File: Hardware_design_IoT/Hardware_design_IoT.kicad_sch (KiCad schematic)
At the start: 0 parts

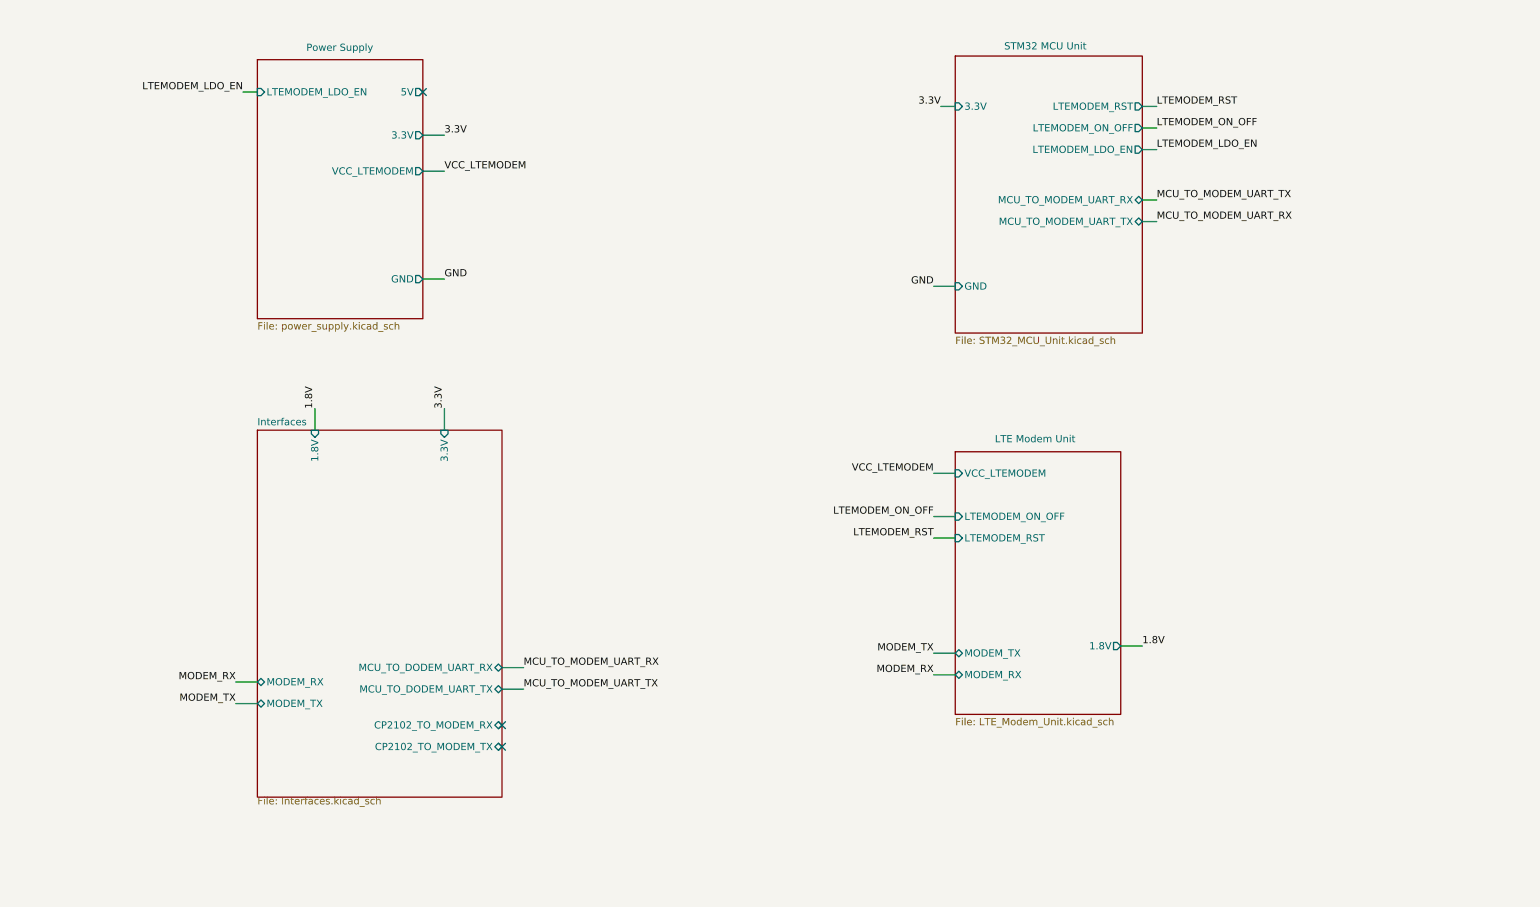
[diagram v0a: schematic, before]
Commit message: Fin du projet
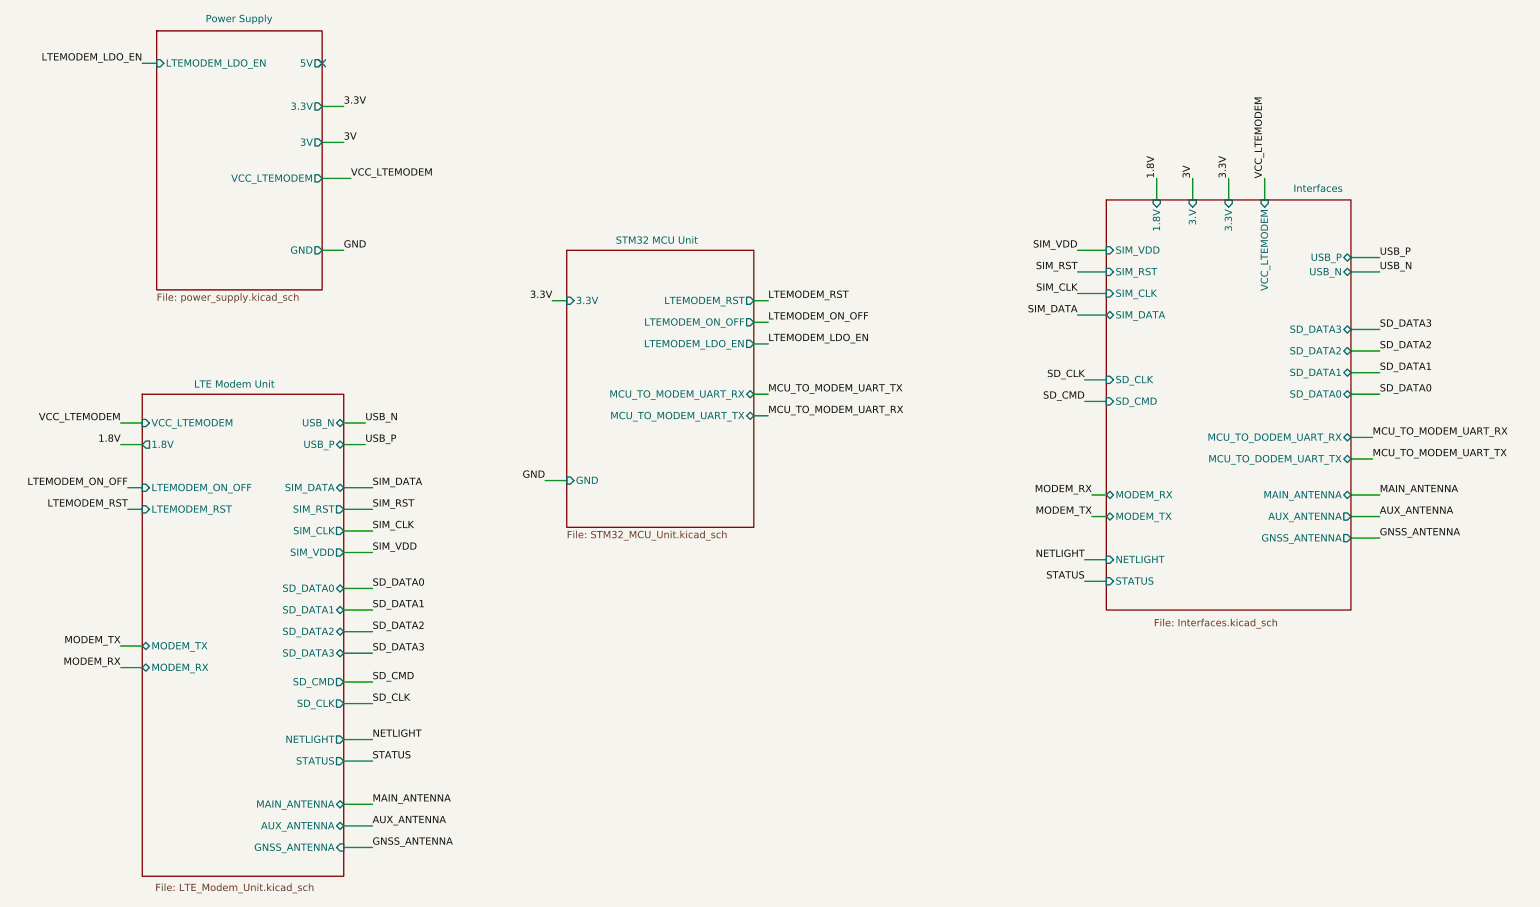
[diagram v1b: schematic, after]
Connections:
- no-connect marks 3 -> 1
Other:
- sheet Interfaces ports: added 3.V, AUX_ANTENNA, GNSS_ANTENNA, MAIN_ANTENNA, NETLIGHT, SD_CLK, SD_CMD, SD_DATA0, SD_DATA1, SD_DATA2, SD_DATA3, SIM_CLK, SIM_DATA, SIM_RST, SIM_VDD, STATUS, USB_N, USB_P, VCC_LTEMODEM; removed CP2102_TO_MODEM_RX, CP2102_TO_MODEM_TX
- sheet LTE Modem Unit ports: added AUX_ANTENNA, GNSS_ANTENNA, MAIN_ANTENNA, NETLIGHT, SD_CLK, SD_CMD, SD_DATA0, SD_DATA1, SD_DATA2, SD_DATA3, SIM_CLK, SIM_DATA, SIM_RST, SIM_VDD, STATUS, USB_N, USB_P; removed none
- sheet Power Supply ports: added 3V; removed none
